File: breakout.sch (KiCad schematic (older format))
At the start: 32 parts, among them CON1 SD_Card, CON2 USB-MICRO-AB, P2 CONN_01X40, P3 CONN_01X40, P4 CONN_01X40, P5 A-DF-09-A/KG-T4S, SW1 SW_PUSH

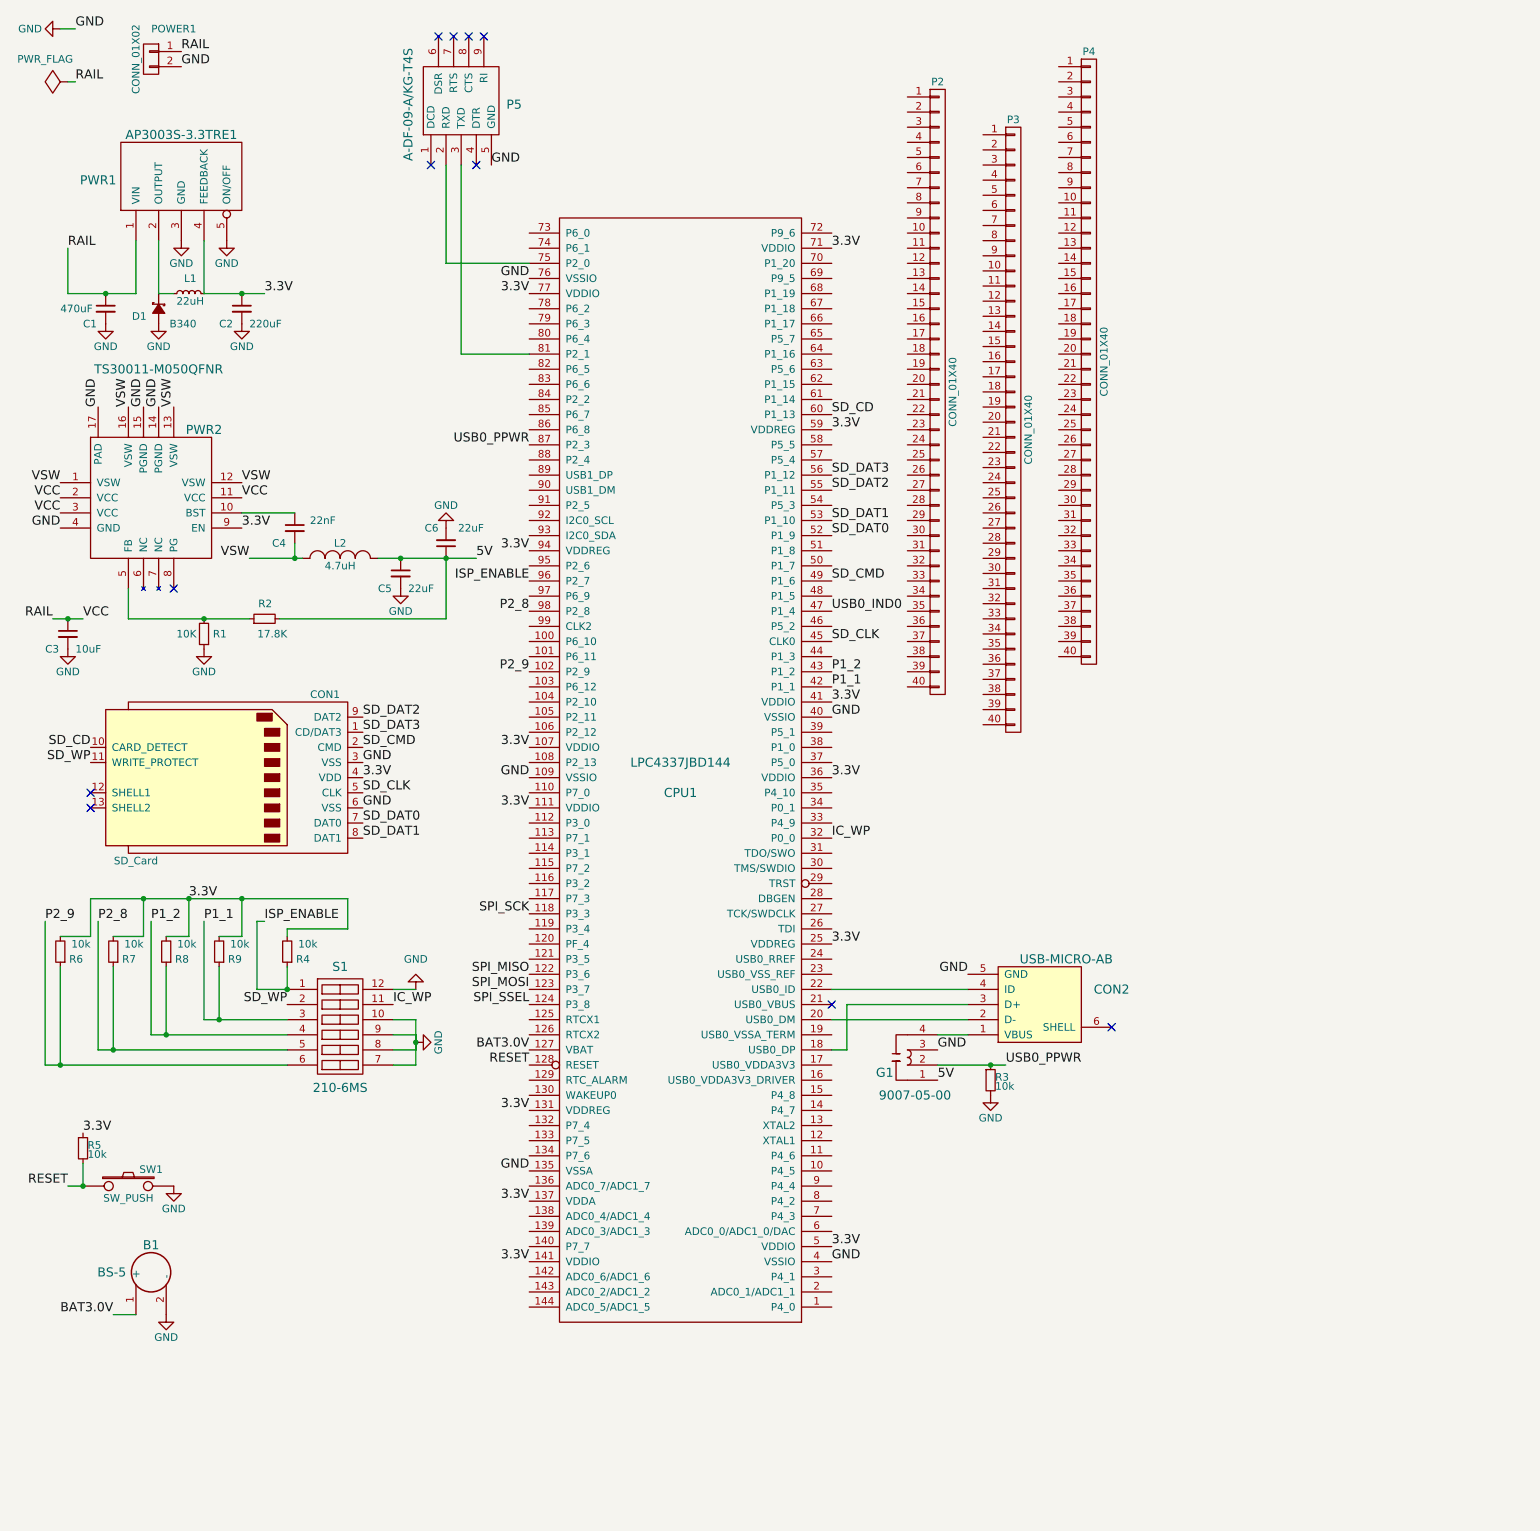
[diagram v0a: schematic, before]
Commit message: fixing net names
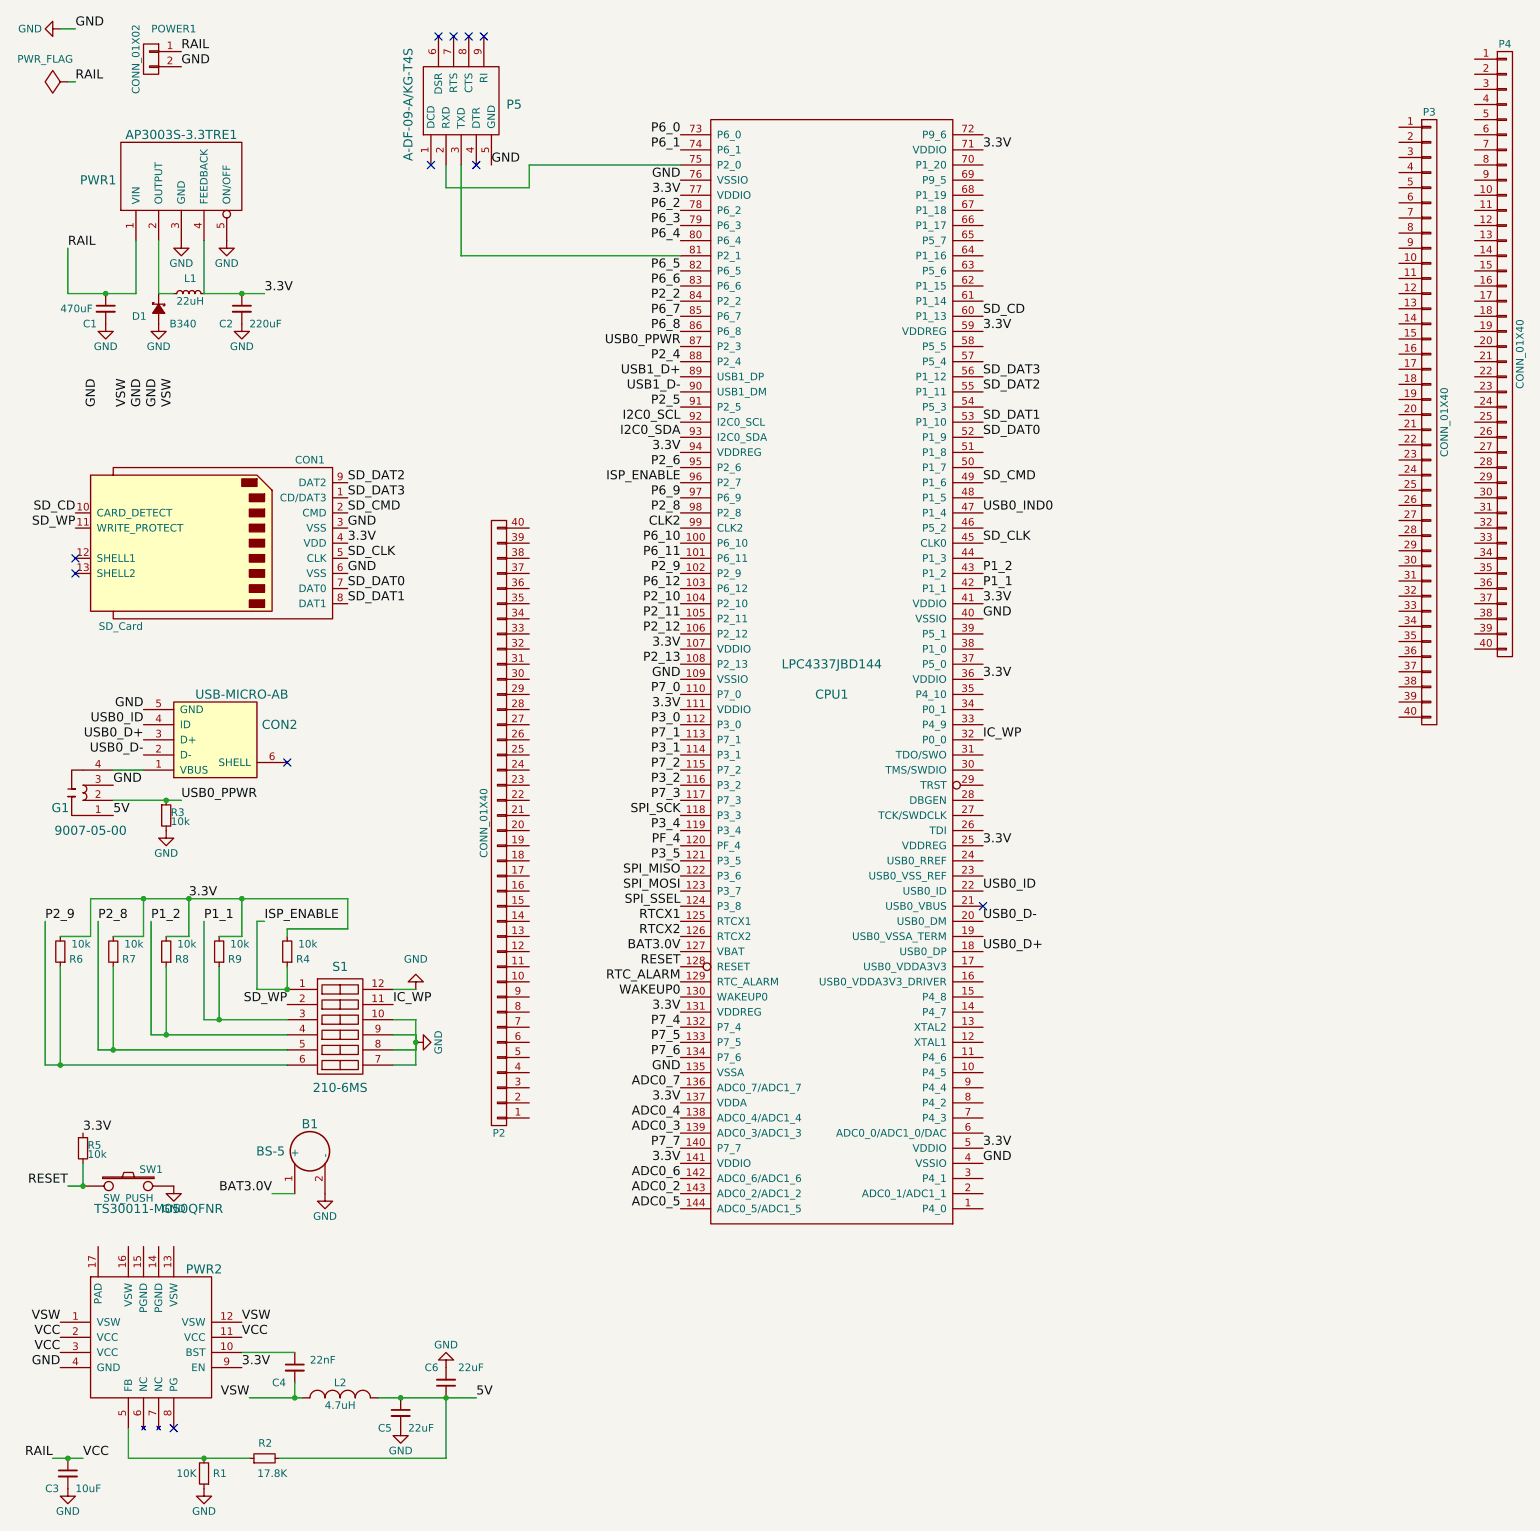
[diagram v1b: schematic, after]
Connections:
- net GND: no longer PWR2.14 (PGND), PWR2.15 (PGND), PWR2.17 (PAD)
- net VSW: no longer PWR2.13 (VSW), PWR2.16 (VSW)
- net P6_10: now reaches CPU1.100 (P6_10)
- net P6_11: now reaches CPU1.101 (P6_11)
- net P6_12: now reaches CPU1.103 (P6_12)
- net P2_10: now reaches CPU1.104 (P2_10)
- net P2_11: now reaches CPU1.105 (P2_11)
- net P2_12: now reaches CPU1.106 (P2_12)
- net P2_13: now reaches CPU1.108 (P2_13)
- net P7_0: now reaches CPU1.110 (P7_0)
- net P3_0: now reaches CPU1.112 (P3_0)
- net P7_1: now reaches CPU1.113 (P7_1)
- net P3_1: now reaches CPU1.114 (P3_1)
- net P7_2: now reaches CPU1.115 (P7_2)
- net P3_2: now reaches CPU1.116 (P3_2)
- net P7_3: now reaches CPU1.117 (P7_3)
- net P3_4: now reaches CPU1.119 (P3_4)
- net PF_4: now reaches CPU1.120 (PF_4)
- net P3_5: now reaches CPU1.121 (P3_5)
- net RTCX1: now reaches CPU1.125 (RTCX1)
- net RTCX2: now reaches CPU1.126 (RTCX2)
- net RTC_ALARM: now reaches CPU1.129 (RTC_ALARM)
- net WAKEUP0: now reaches CPU1.130 (WAKEUP0)
- net P7_4: now reaches CPU1.132 (P7_4)
- net P7_5: now reaches CPU1.133 (P7_5)
- net P7_6: now reaches CPU1.134 (P7_6)
- net ADC0_7: now reaches CPU1.136 (ADC0_7/ADC1_7)
- net ADC0_4: now reaches CPU1.138 (ADC0_4/ADC1_4)
- net ADC0_3: now reaches CPU1.139 (ADC0_3/ADC1_3)
- net P7_7: now reaches CPU1.140 (P7_7)
- net ADC0_6: now reaches CPU1.142 (ADC0_6/ADC1_6)
- net ADC0_2: now reaches CPU1.143 (ADC0_2/ADC1_2)
- net ADC0_5: now reaches CPU1.144 (ADC0_5/ADC1_5)
- net USB0_D+: now reaches CON2.3 (D+), CPU1.18 (USB0_DP)
- net USB0_D-: now reaches CON2.2 (D-), CPU1.20 (USB0_DM)
- net USB0_ID: now reaches CON2.4 (ID), CPU1.22 (USB0_ID)
- net P6_0: now reaches CPU1.73 (P6_0)
- net P6_1: now reaches CPU1.74 (P6_1)
- net P6_2: now reaches CPU1.78 (P6_2)
- net P6_3: now reaches CPU1.79 (P6_3)
- net P6_4: now reaches CPU1.80 (P6_4)
- net P6_5: now reaches CPU1.82 (P6_5)
- net P6_6: now reaches CPU1.83 (P6_6)
- net P2_2: now reaches CPU1.84 (P2_2)
- net P6_7: now reaches CPU1.85 (P6_7)
- net P6_8: now reaches CPU1.86 (P6_8)
- net P2_4: now reaches CPU1.88 (P2_4)
- net USB1_D+: now reaches CPU1.89 (USB1_DP)
- net USB1_D-: now reaches CPU1.90 (USB1_DM)
- net P2_5: now reaches CPU1.91 (P2_5)
- net I2C0_SCL: now reaches CPU1.92 (I2C0_SCL)
- net I2C0_SDA: now reaches CPU1.93 (I2C0_SDA)
- net P2_6: now reaches CPU1.95 (P2_6)
- net P6_9: now reaches CPU1.97 (P6_9)
- net CLK2: now reaches CPU1.99 (CLK2)
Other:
- moved on the sheet: B1, C3, C4, C5, C6, CON1, CON2, CPU1, G1, L2, P2, P3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
